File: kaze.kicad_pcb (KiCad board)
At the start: 2 copper layers, 40 x 22.1 mm, 42 parts, among them J1 Conn_01x02_Pin, P1 USB_C_Plug_USB2.0, SW1 SW_Push, SW2 SW_Push, U1 MCP73831-2-OT, U2 BME680, U3 AP2112K-3.3, U4 ESP32-C6-MINI-1, U5 TSL25911FN

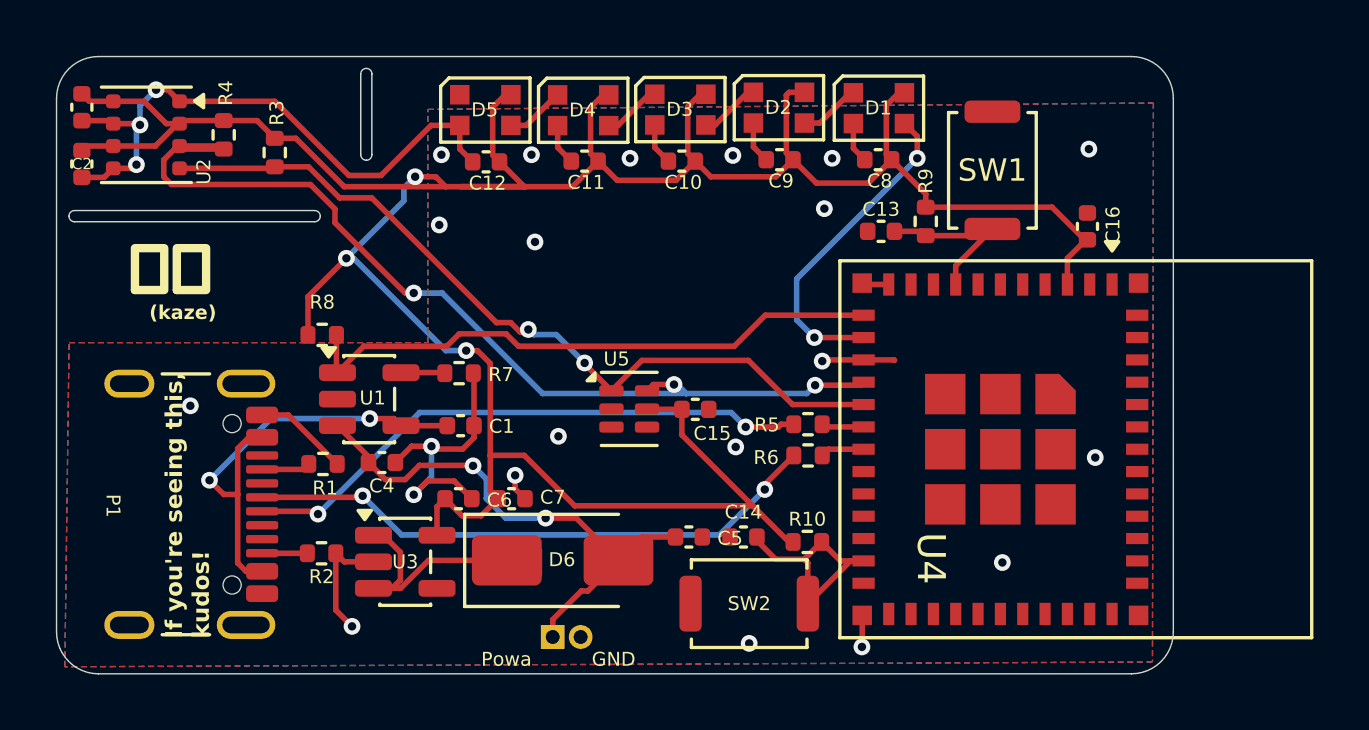
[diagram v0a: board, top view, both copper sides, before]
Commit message: pcb
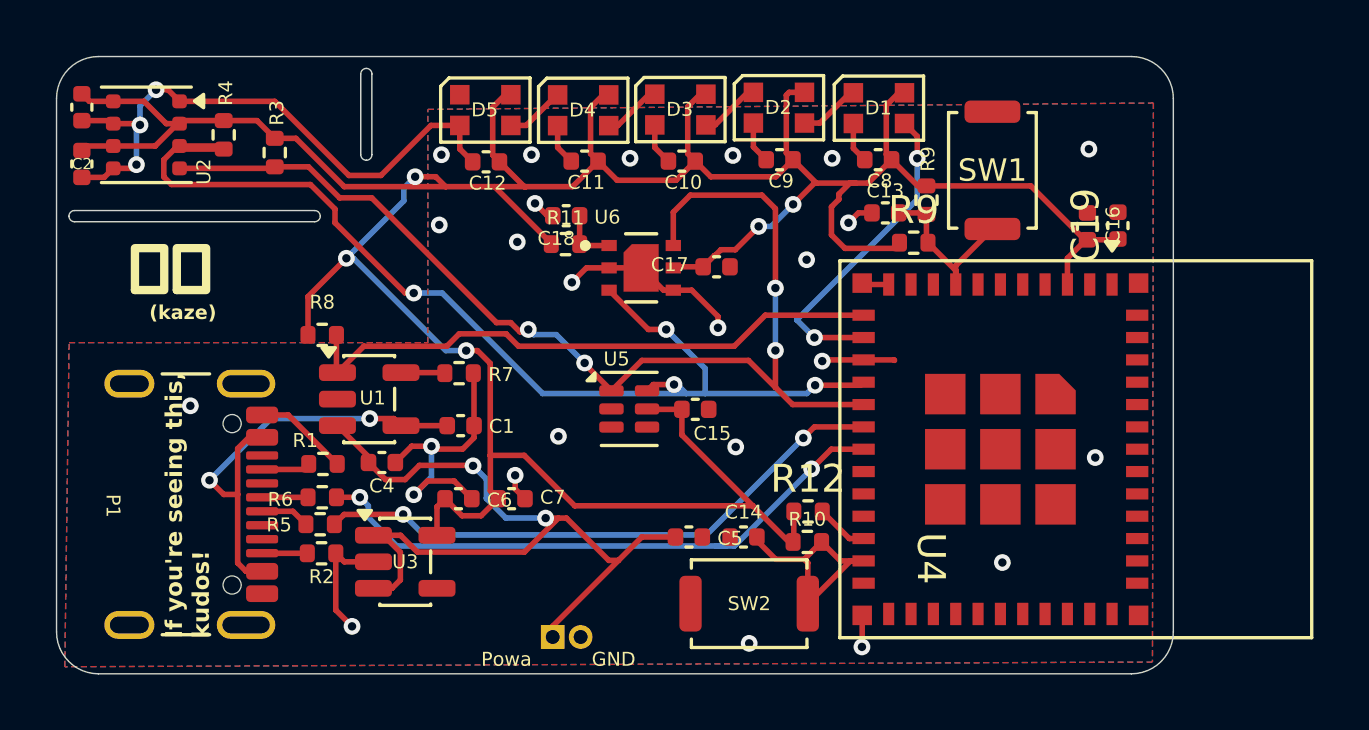
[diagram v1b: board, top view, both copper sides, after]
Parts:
- removed D6: SS14, Diode_SMD:D_SMA
- removed the R9 at (177.1, 74.3)
- added C17: 1uF, Capacitor_SMD:C_0402_1005Metric, F.Cu at (169.6, 75.9)
- added C18: 1uF, Capacitor_SMD:C_0402_1005Metric, F.Cu at (164.2, 74.1)
- added C19: 22uf, Capacitor_SMD:C_0402_1005Metric, F.Cu at (184.0, 74.4)
- added R11: 4.7, Resistor_SMD:R_0402_1005Metric, F.Cu at (164.2, 75.1)
- added R12: 10k, Resistor_SMD:R_0402_1005Metric, F.Cu at (172.9, 84.7)
- added R9: 10k, Resistor_SMD:R_0402_1005Metric, F.Cu at (176.7, 75.1)
- added R9: 10k, Resistor_SMD:R_0402_1005Metric, F.Cu at (177.1, 73.5)
- added U6: SGP40-D-R4, SGP40_D_R4:XCDR_SGP40-D-R4, F.Cu at (166.9, 76.0)
- C13: value 10uF -> 1uF
- moved R5 17.8 mm to (155.4, 85.1)
- moved R6 17.5 mm to (155.5, 84.2)
- moved C13 0.68 mm to (175.6, 74.0)
- moved G*** 0.11 mm to (166.0, 79.4)
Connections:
- U3 pad 1: Net-(D6-K) -> +BATT
- U3 pad 3: Net-(D6-K) -> +BATT
- U4 pad 22: unconnected-(U4-IO8-Pad22) -> Net-(U4-IO8)
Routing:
- net /D+: track 1.57 -> 21.7 mm, vias 0 -> 2
- net /D-: track 1.52 -> 21.0 mm, vias 0 -> 2
- net Net-(P1-D+): track 20.9 -> 1.64 mm, vias 2 -> 0
- net Net-(P1-D-): track 20.8 -> 1.76 mm, vias 2 -> 0
- net +3V3: track 107.0 -> 121.2 mm, vias 3 -> 5
- net /SCL: track 29.0 -> 40.7 mm, vias 2 -> 4
- net +BATT: track 19.3 -> 29.8 mm
- net Net-(D6-K): track 9.38 -> 0.00 mm
- net GND: track 51.3 -> 59.6 mm, vias 24 -> 28
- net /SDA: track 35.0 -> 40.5 mm, vias 3 -> 4
- net Net-(U6-VDD): track 0.00 -> 2.09 mm
- net Net-(U4-IO8): track 0.00 -> 1.88 mm
- net /EN: track 6.20 -> 6.83 mm
